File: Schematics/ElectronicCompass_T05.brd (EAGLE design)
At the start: 50.5 x 50.8 mm, 67 parts, among them Q1 FDN360P, Q2 FDN360P, Q3 FDN360P, Q4 FDN360P, Q5 BC817-16LT1SMD, Q6 BC817-16LT1SMD, U1 ATMEGA32U4, X1 USBSMD, Y1 16MHz

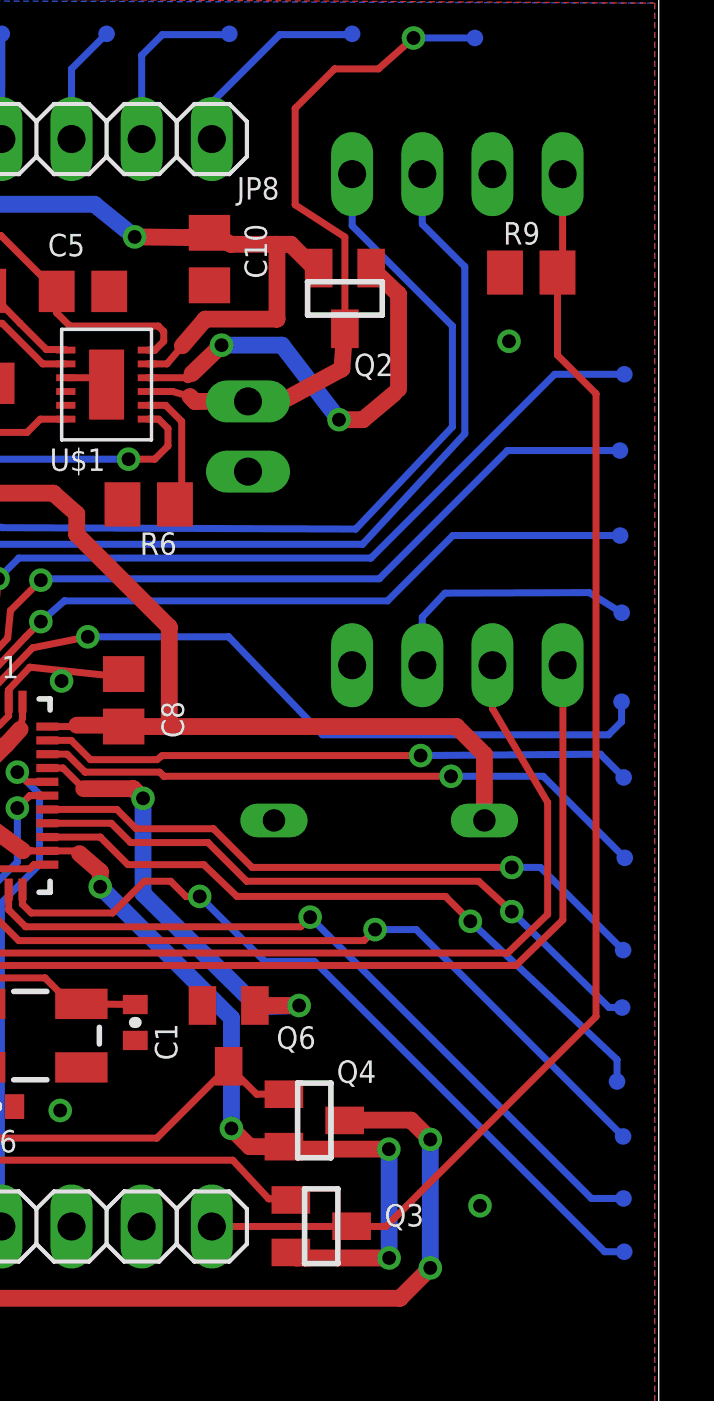
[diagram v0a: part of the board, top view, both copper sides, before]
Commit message: layout update
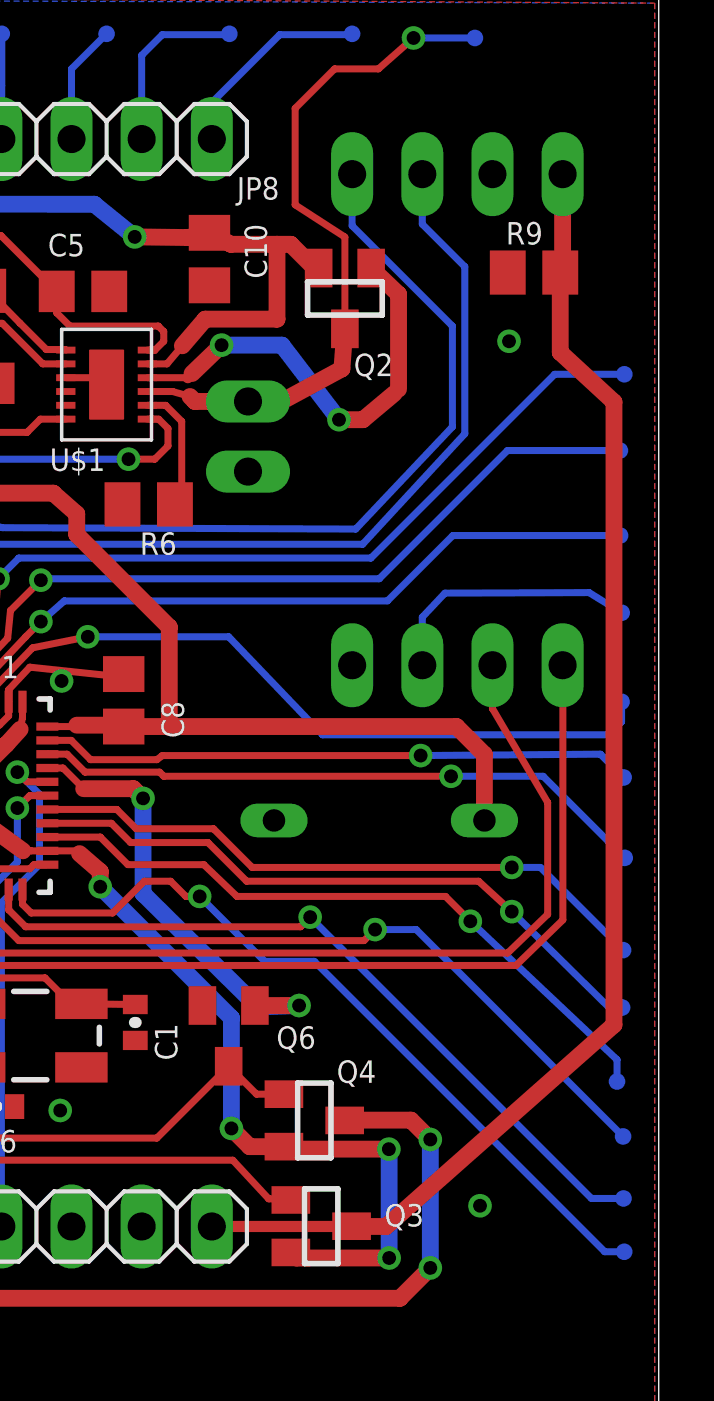
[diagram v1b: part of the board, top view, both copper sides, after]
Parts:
- moved R9 0.10 mm to (46.0, 40.9)
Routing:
- net VCC': track 48.3 -> 49.0 mm
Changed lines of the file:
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@@
 <attribute name="VALUE" x="23.511" y="13.6935" size="0.8128" layer="27" rot="R180"/>
 </element>
-<element name="R9" library="resistor" package="M0805" value="1k" x="45.855" y="40.88625" smashed="yes">
-<attribute name="NAME" x="44.839" y="41.90225" size="0.8128" layer="25"/>
-<attribute name="VALUE" x="44.839" y="38.60025" size="0.8128" layer="27"/>
+<element name="R9" library="resistor" package="M0805" value="1k" x="45.955" y="40.88625" smashed="yes">
+<attribute name="NAME" x="44.939" y="41.90225" size="0.8128" layer="25"/>
+<attribute name="VALUE" x="44.939" y="38.60025" size="0.8128" layer="27"/>
 </element>
 <element name="R10" library="resistor" package="M0805" value="1M" x="19.18" y="10.495" smashed="yes" rot="R270">
@@
 <contactref element="R9" pad="2"/>
 <contactref element="Q3" pad="3"/>
-<wire x1="34.29" y1="6.35" x2="39.31" y2="6.35" width="0.254" layer="1"/>
+<wire x1="34.29" y1="6.35" x2="39.31" y2="6.35" width="0.4064" layer="1"/>
 <wire x1="39.31" y1="6.35" x2="39.35" y2="6.36" width="0.254" layer="1"/>
-<wire x1="39.31" y1="6.35" x2="40.6" y2="6.35" width="0.254" layer="1"/>
-<wire x1="40.6" y1="6.35" x2="48.2" y2="13.95" width="0.254" layer="1"/>
-<wire x1="46.99" y1="44.45" x2="46.99" y2="41.07125" width="0.254" layer="1"/>
-<wire x1="46.99" y1="41.07125" x2="46.805" y2="40.88625" width="0.254" layer="1"/>
-<wire x1="46.805" y1="40.88625" x2="46.805" y2="37.895" width="0.254" layer="1"/>
-<wire x1="46.805" y1="37.895" x2="48.2" y2="36.5" width="0.254" layer="1"/>
-<wire x1="48.2" y1="36.5" x2="48.2" y2="13.95" width="0.254" layer="1"/>
+<wire x1="39.31" y1="6.35" x2="40.6" y2="6.35" width="0.6096" layer="1"/>
+<wire x1="40.6" y1="6.35" x2="48.85" y2="13.65" width="0.6096" layer="1"/>
+<wire x1="46.99" y1="44.45" x2="46.99" y2="41.07125" width="0.6096" layer="1"/>
+<wire x1="46.99" y1="41.07125" x2="46.905" y2="40.88625" width="0.254" layer="1"/>
+<wire x1="46.905" y1="40.88625" x2="46.905" y2="37.995" width="0.6096" layer="1"/>
+<wire x1="46.905" y1="37.995" x2="48.85" y2="36.2" width="0.6096" layer="1"/>
+<wire x1="48.85" y1="36.2" x2="48.85" y2="13.65" width="0.6096" layer="1"/>
 </signal>
 <signal name="RESET">
